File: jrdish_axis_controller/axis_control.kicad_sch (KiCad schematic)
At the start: 30 parts, among them CN7 KF2EDGR-2.54-9P, CN8 KF2EDGR-2.54-6P, U3 LTV-847S, U5 LTV-827S-TA1, U6 LTV-817S-TA1, U7 LTV-817S-TA1

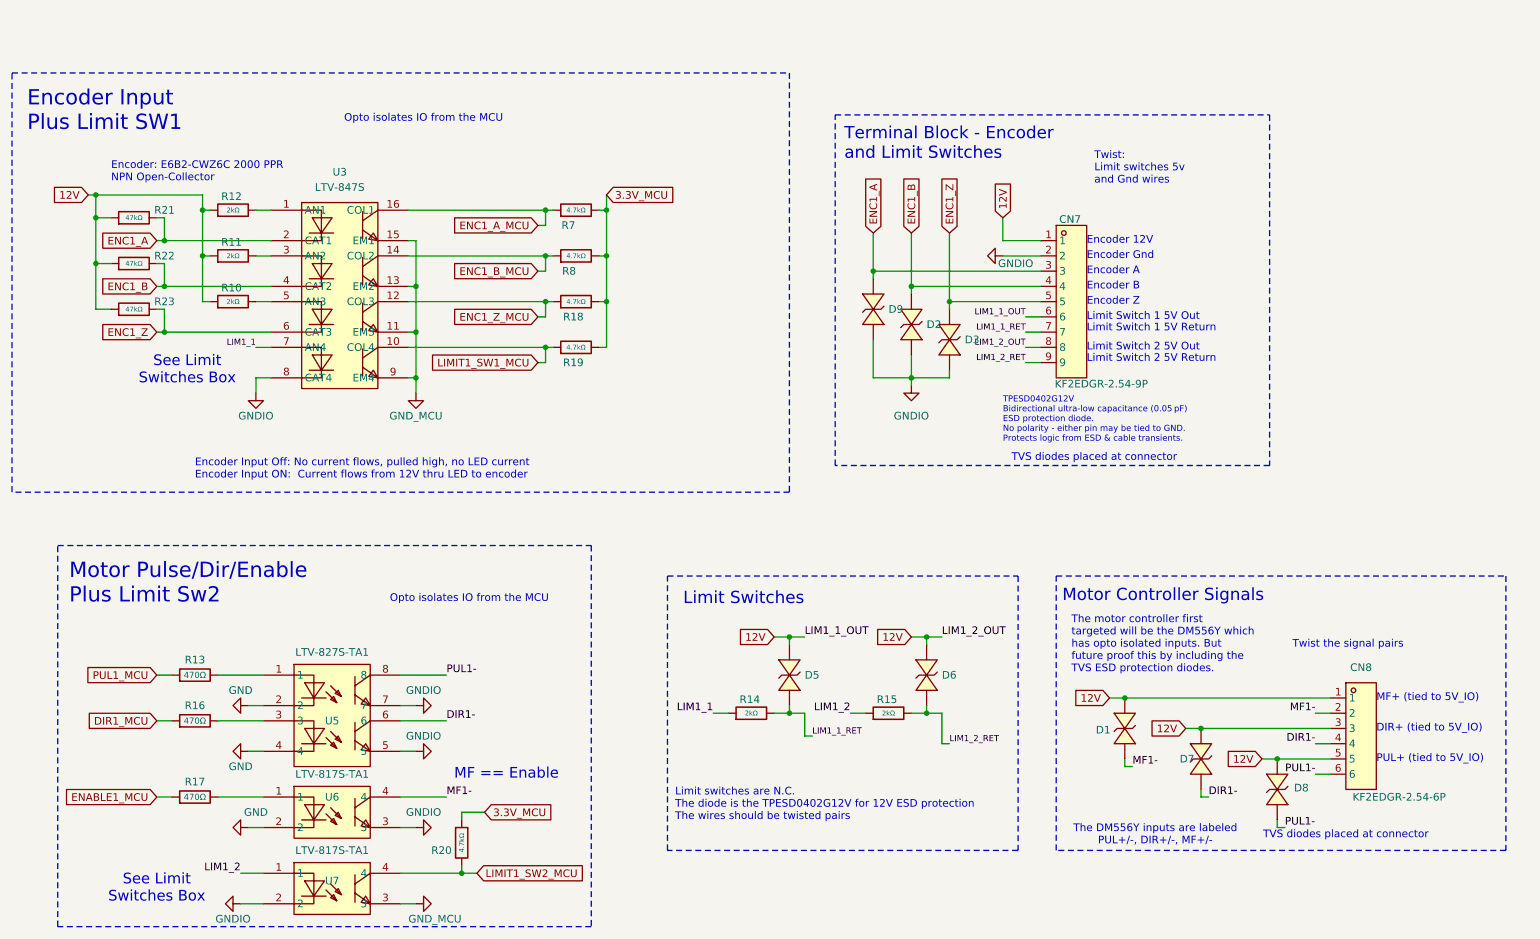
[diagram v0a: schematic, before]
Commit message: Updates
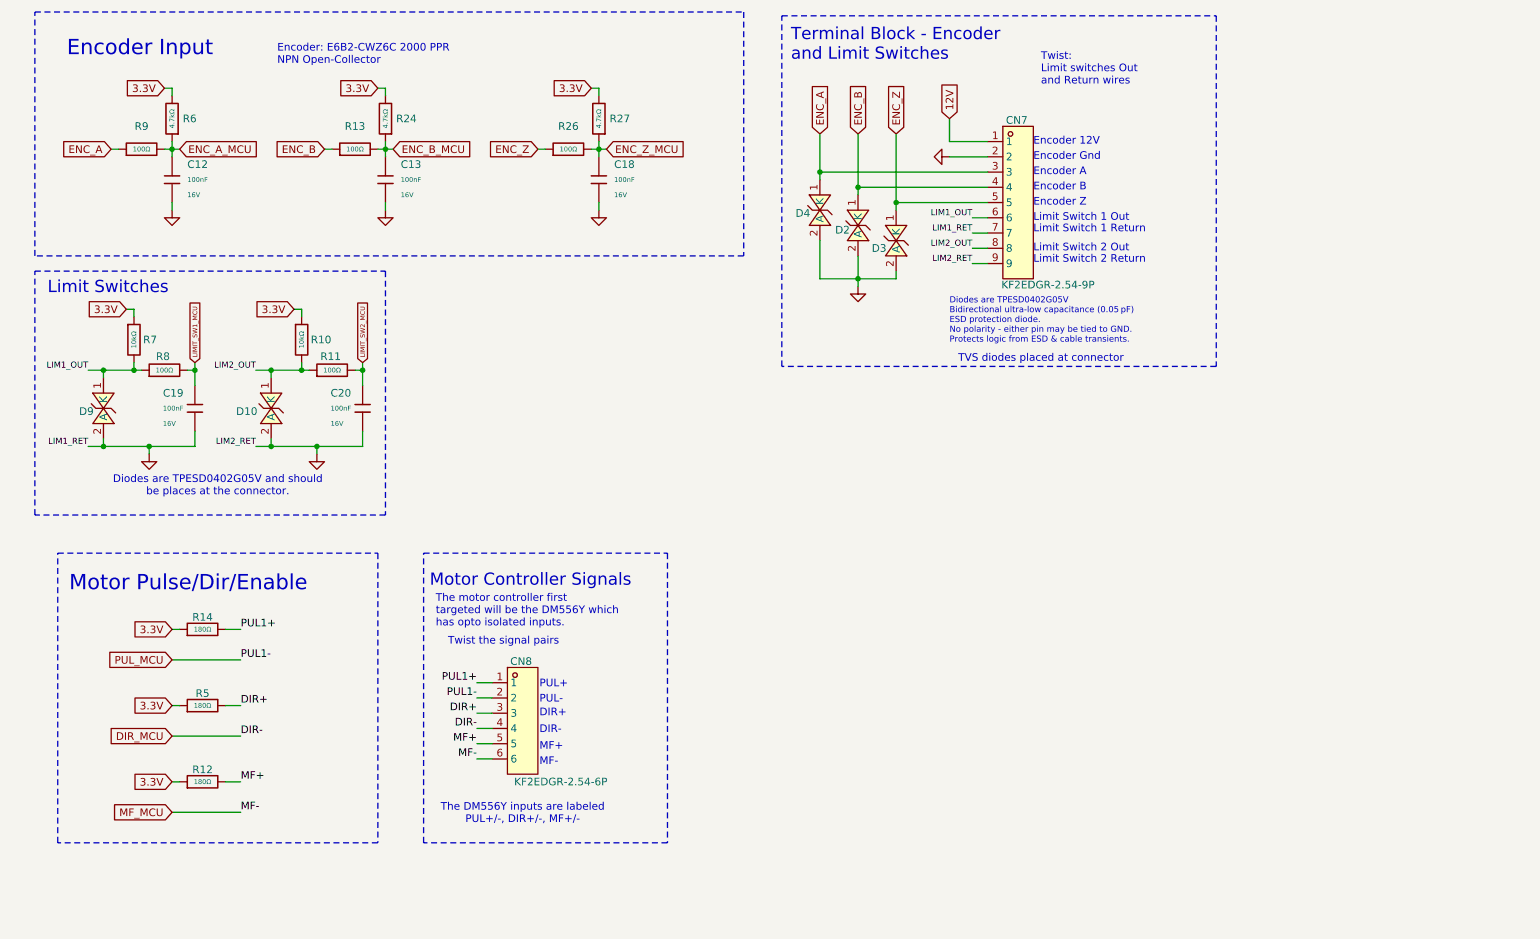
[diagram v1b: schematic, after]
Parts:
- removed D1, D2, D3, D5, D6, D7, D8, D9: TPESD0402G12V, MyParts:D0402-BI, symbol MyParts:TPESD0402G12V
- removed R10, R11, R12, R14, R15: 2kΩ, PCM_JLCPCB:R_0402, symbol PCM_JLCPCB-Resistors:0402,2kΩ
- removed R13, R16, R17: 470Ω, PCM_JLCPCB:R_0402, symbol PCM_JLCPCB-Resistors:0402,470Ω
- removed R18, R19, R20, R7, R8: 4.7kΩ, PCM_JLCPCB:R_0603, symbol PCM_JLCPCB-Resistors:0603,4.7kΩ
- removed R21, R22, R23: 47kΩ, PCM_JLCPCB:R_0402, symbol PCM_JLCPCB-Resistors:0402,47kΩ
- removed U3: LTV-847S, MyParts:SMD-16_L20.0-W6.5-P2.54-LS10.2-BL, symbol MyParts:LTV-847S
- removed U5: LTV-827S-TA1, MyParts:SMD-8_L9.8-W6.6-P2.54-LS10.3-BL, symbol MyParts:LTV-827S-TA1
- removed U6, U7: LTV-817S-TA1, MyParts:OPTO-SMD-4_L4.6-W6.5-P2.54-LS10.3-BL, symbol MyParts:LTV-817S-TA1
- added C12, C13, C18, C19, C20: 100nF, PCM_JLCPCB:C_0402, symbol PCM_JLCPCB-Capacitors:0402,100nF
- added D10, D2, D3, D4, D9: TPESD0402G05V, MyParts:D0402-BI, symbol MyParts:TPESD0402G05V
- added R10, R7: 10kΩ, PCM_JLCPCB:R_0402, symbol PCM_JLCPCB-Resistors:0402,10kΩ
- added R11, R13, R26, R8, R9: 100Ω, PCM_JLCPCB:R_0402, symbol PCM_JLCPCB-Resistors:0402,100Ω
- added R12, R14, R5: 180Ω, PCM_JLCPCB:R_0603, symbol PCM_JLCPCB-Resistors:0603,180Ω
- added R24, R27, R6: 4.7kΩ, PCM_JLCPCB:R_0402, symbol PCM_JLCPCB-Resistors:0402,4.7kΩ
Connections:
- net GNDIO is gone; now on net GND: CN7.2
- net LIM1_1_RET is gone; now on net GND: CN7.7
- net LIM1_2_RET is gone; now on net GND: CN7.9
- net 12V: no longer CN7.6, CN7.8, CN8.1, CN8.3, CN8.5
- net GND: now also C12.2, C13.2, C18.2, C19.2, C20.2, D10.2 (A), D2.2 (A), D3.2 (A), D4.2 (A), D9.2 (A)
- net DIR1- renamed DIR_MCU
- net ENC1_A renamed ENC_A
- net ENC_A: now also D4.1 (K), R9.1
- net ENC1_B renamed ENC_B
- net ENC_B: now also D2.1 (K), R13.1
- net ENC1_Z renamed ENC_Z
- net ENC_Z: now also D3.1 (K), R26.1
- net MF1- renamed PUL_MCU
- net PUL1- renamed MF_MCU
- new net 3.3V: R10.1, R12.1, R14.1, R24.2, R27.2, R5.1, R6.2, R7.1
- new net DIR+: CN8.3, R5.2
- new net ENC_A_MCU: C12.1, R6.1, R9.2
- new net ENC_B_MCU: C13.1, R13.2, R24.1
- new net ENC_Z_MCU: C18.1, R26.2, R27.1
- new net LIM1_OUT: CN7.6, D9.1 (K), R7.2, R8.1
- new net LIM2_OUT: CN7.8, D10.1 (K), R10.2, R11.1
- new net LIMIT_SW1_MCU: C19.1, R8.2
- new net LIMIT_SW2_MCU: C20.1, R11.2
- new net MF+: CN8.5, R12.2
- new net PUL1+: CN8.1, R14.2
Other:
- note added: "DIR+"
- note added: "DIR-"
- note added: "Diodes are TPESD0402G05V Bidirectional ultra-low capacitance (0.05 pF) ESD protection diode. No polarity - either pin may be tied to GND. Protects logic from ESD & cable transients."
- note added: "Diodes are TPESD0402G05V and should be places at the connector."
- note added: "Encoder Input"
- note added: "Limit Switch 1 Out"
- note added: "Limit Switch 1 Return"
- note added: "Limit Switch 2 Out"
- note added: "Limit Switch 2 Return"
- note added: "MF+"
- note added: "MF-"
- note added: "Motor Pulse/Dir/Enable"
- note added: "PUL+"
- note added: "PUL-"
- note added: "The motor controller first targeted will be the DM556Y which has opto isolated inputs."
- note added: "Twist: Limit switches Out and Return wires"
- note removed: "DIR+ (tied to 5V_IO)"
- note removed: "Encoder Input Off: No current flows, pulled high, no LED current Encoder Input ON: Current flows from 12V thru LED to encoder"
- note removed: "Encoder Input Plus Limit SW1"
- note removed: "Limit Switch 1 5V Out"
- note removed: "Limit Switch 1 5V Return"
- note removed: "Limit Switch 2 5V Out"
- note removed: "Limit Switch 2 5V Return"
- note removed: "Limit switches are N.C. The diode is the TPESD0402G12V for 12V ESD protection The wires should be twisted pairs"
- note removed: "MF == Enable"
- note removed: "MF+ (tied to 5V_IO)"
- note removed: "Motor Pulse/Dir/Enable Plus Limit Sw2"
- note removed: "Opto isolates IO from the MCU"
- note removed: "PUL+ (tied to 5V_IO)"
- note removed: "See Limit Switches Box"
- note removed: "TPESD0402G12V Bidirectional ultra-low capacitance (0.05 pF) ESD protection diode. No polarity - either pin may be tied to GND. Protects logic from ESD & cable transients."
- note removed: "The motor controller first targeted will be the DM556Y which has opto isolated inputs. But future proof this by including the TVS ESD protection diodes."
- note removed: "Twist: Limit switches 5v and Gnd wires"
- moved on the sheet: CN7, CN8
